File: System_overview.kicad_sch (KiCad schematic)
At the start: 0 parts

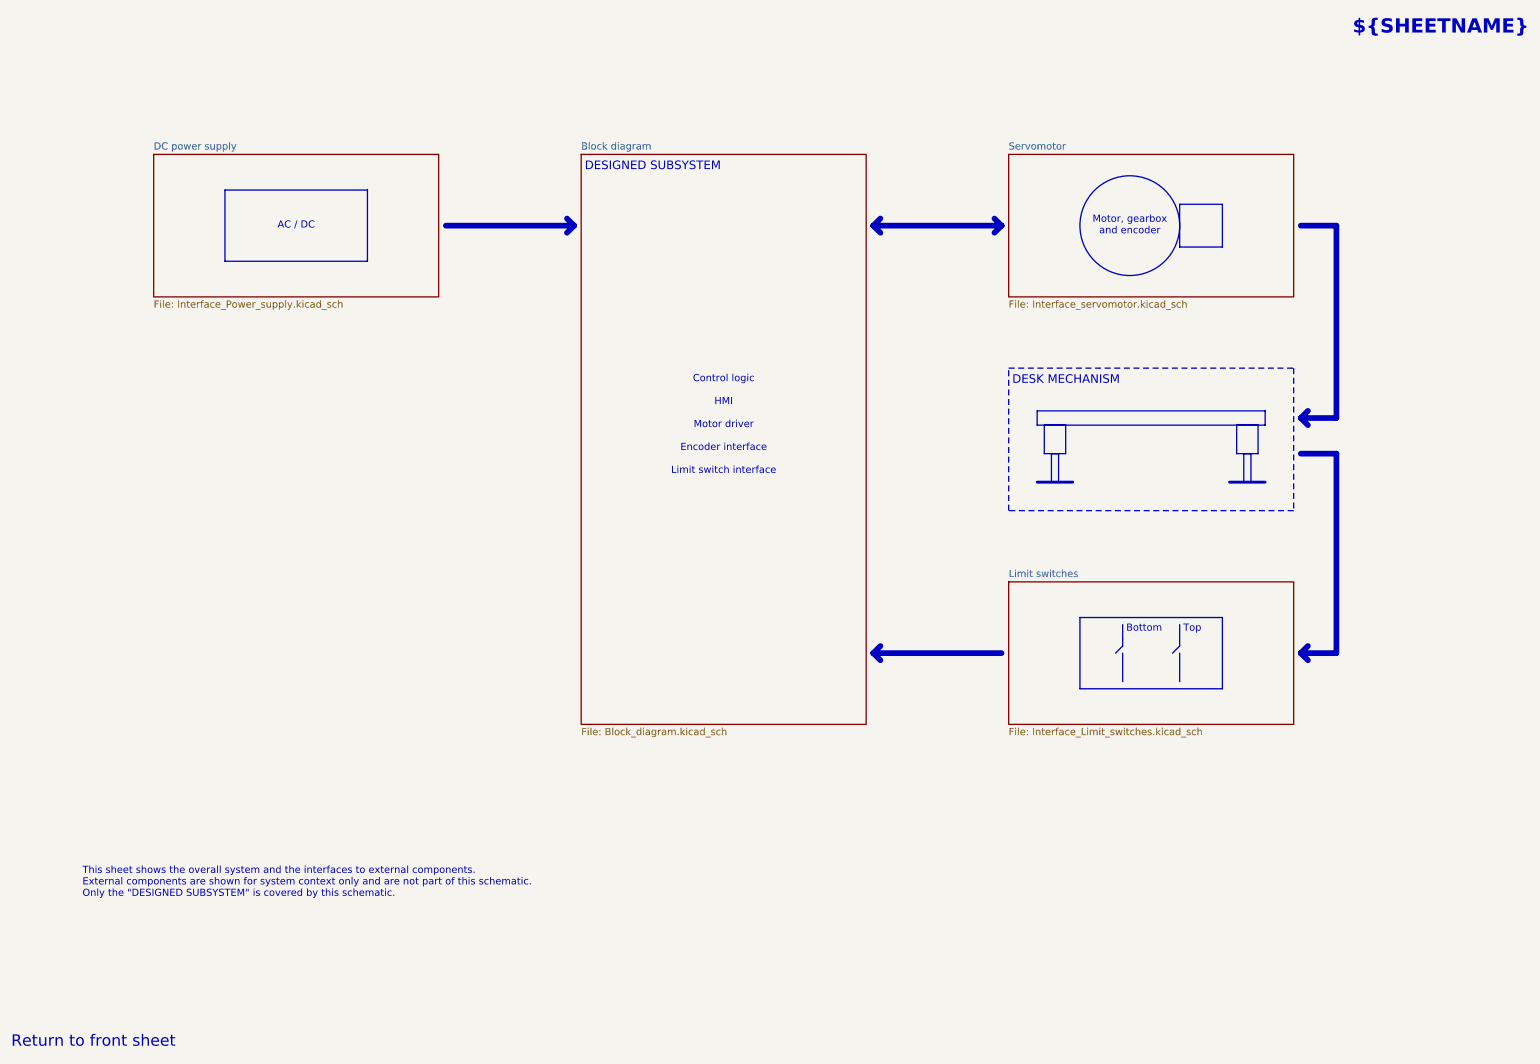
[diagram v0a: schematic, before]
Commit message: testing green mask
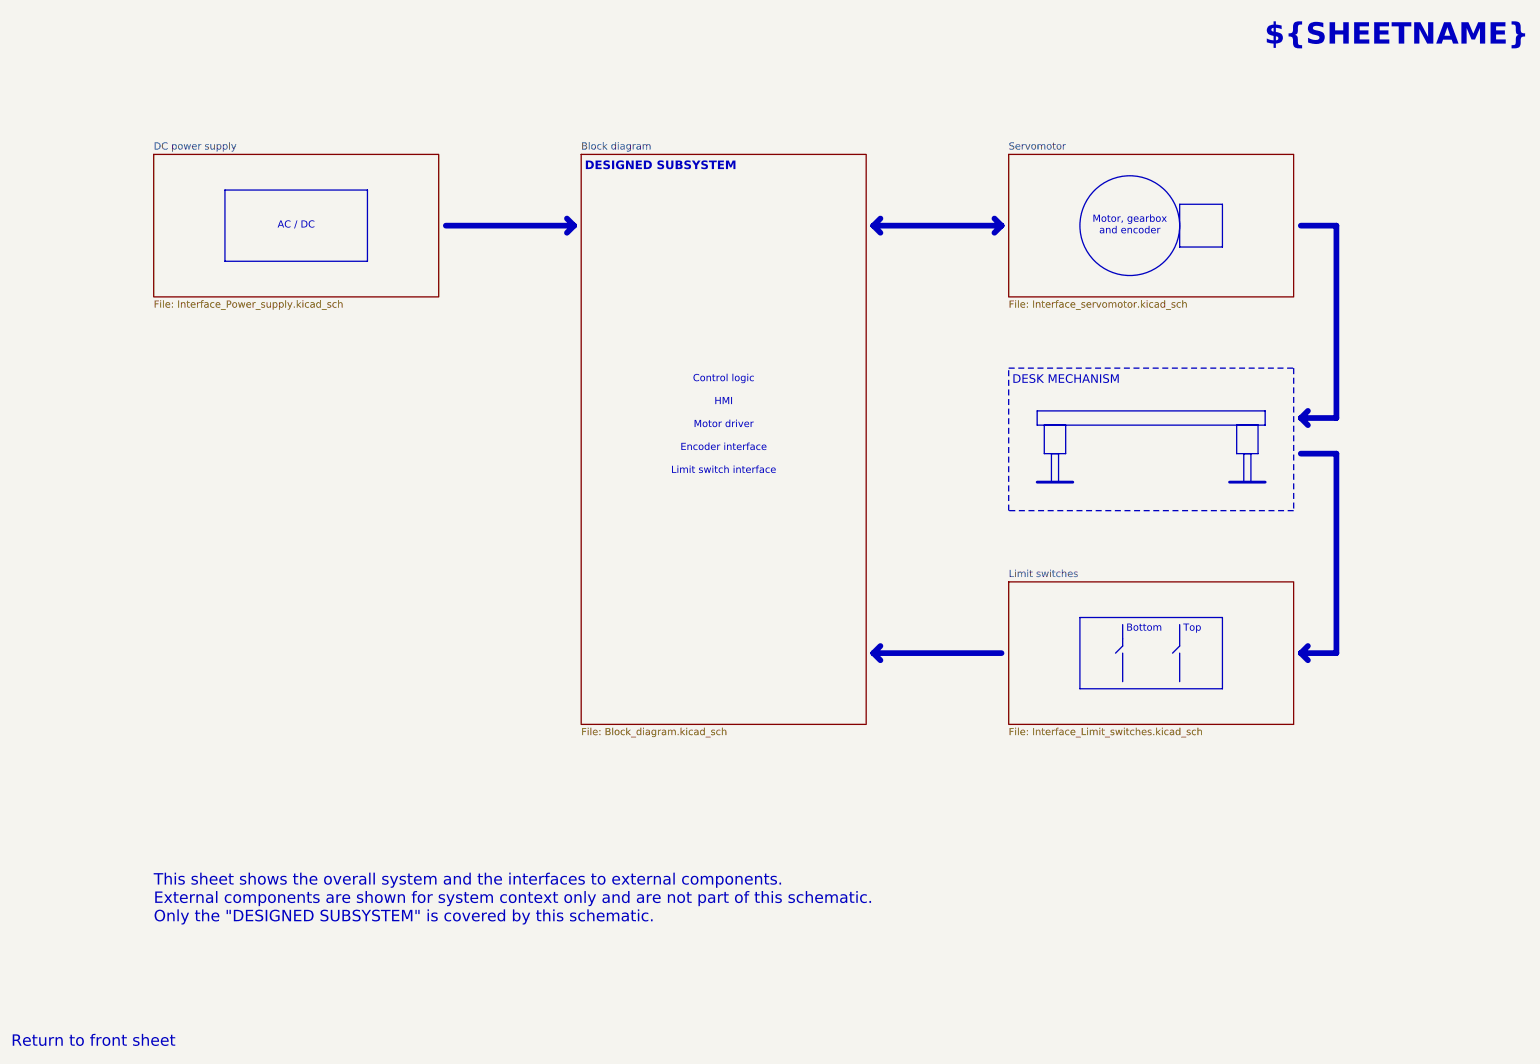
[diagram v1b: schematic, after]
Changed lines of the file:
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@@
 			(width 0)
 			(type dash)
+			(color 0 0 0 1)
 		)
 		(fill
@@
 	(text "This sheet shows the overall system and the interfaces to external components.\nExternal components are shown for system context only and are not part of this schematic.\nOnly the \"DESIGNED SUBSYSTEM\" is covered by this schematic."
 		(exclude_from_sim no)
-		(at 25.4 165.1 0)
+		(at 38.1 166.37 0)
 		(effects
 			(font
-				(size 1.27 1.27)
+				(size 2.032 2.032)
+				(color 194 0 0 1)
 			)
 			(justify left top)
@@
 			(font
 				(size 1.27 1.27)
+				(color 0 0 0 1)
 			)
 		)
@@
 				(size 1.524 1.524)
 				(thickness 0.1905)
+				(bold yes)
+				(color 255 0 0 1)
 			)
 			(justify left top)
@@
 	(text "${SHEETNAME}"
 		(exclude_from_sim no)
-		(at 283.21 13.97 0)
+		(at 283.21 14.605 0)
 		(effects
 			(font
-				(size 2.54 2.54)
+				(face "DejaVu Sans")
+				(size 3.81 3.81)
 				(bold yes)
+				(color 0 0 0 1)
 			)
 			(justify right top)
